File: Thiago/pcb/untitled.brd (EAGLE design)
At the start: 87.1 x 59.9 mm, 22 parts, among them IC1 LM358N, J3 -, J5 -

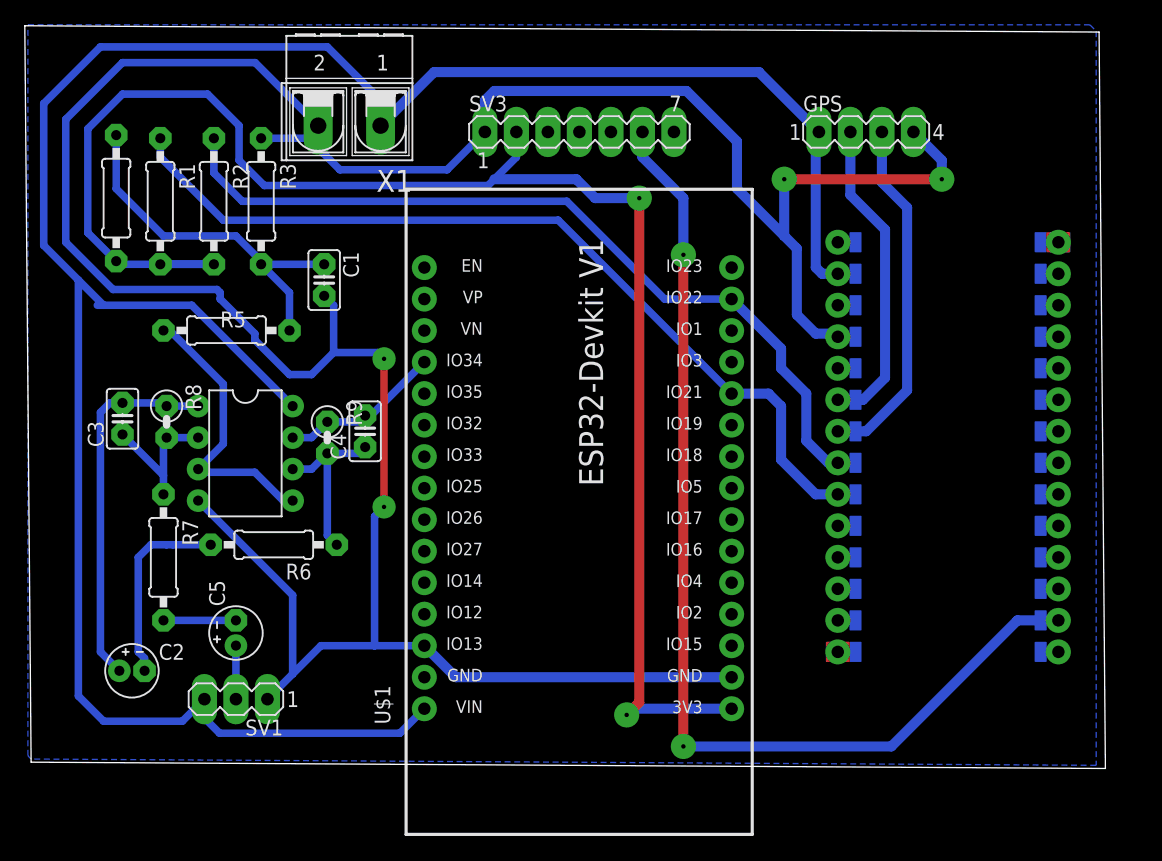
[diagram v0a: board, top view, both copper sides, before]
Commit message: Corrigi espaçãmento pcb
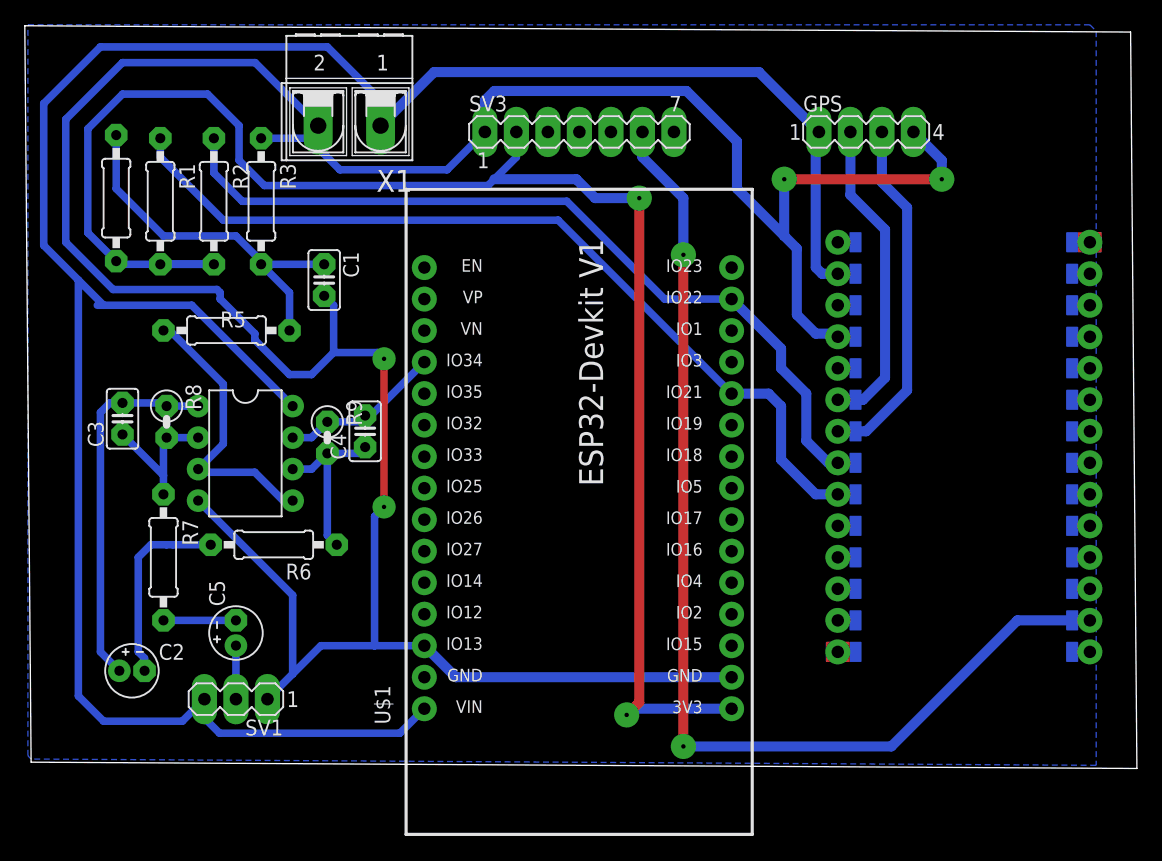
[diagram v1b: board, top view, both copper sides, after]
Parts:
- moved J3 2.54 mm to (100.3, 83.8)
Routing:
- net PWM_OUT: track 85.3 -> 87.9 mm
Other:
- board size 87.1 x 59.9 mm -> 89.6 x 59.9 mm
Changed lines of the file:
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@@
 <setting verticaltext="up"/>
 </settings>
-<grid distance="10" unitdist="mil" unit="mil" style="lines" multiple="1" display="no" altdistance="5" altunitdist="mil" altunit="mil"/>
+<grid distance="0.1" unitdist="mm" unit="mm" style="lines" multiple="1" display="no" altdistance="5" altunitdist="mil" altunit="mil"/>
 <layers>
-<layer number="1" name="Top" color="4" fill="1" visible="yes" active="yes"/>
+<layer number="1" name="Top" color="4" fill="1" visible="no" active="yes"/>
 <layer number="2" name="Route2" color="16" fill="1" visible="no" active="no"/>
 <layer number="3" name="Route3" color="17" fill="1" visible="no" active="no"/>
@@
 <layer number="17" name="Pads" color="2" fill="1" visible="yes" active="yes"/>
 <layer number="18" name="Vias" color="2" fill="1" visible="yes" active="yes"/>
-<layer number="19" name="Unrouted" color="6" fill="1" visible="yes" active="yes"/>
-<layer number="20" name="Dimension" color="24" fill="1" visible="yes" active="yes"/>
-<layer number="21" name="tPlace" color="7" fill="1" visible="yes" active="yes"/>
+<layer number="19" name="Unrouted" color="6" fill="1" visible="no" active="yes"/>
+<layer number="20" name="Dimension" color="24" fill="1" visible="no" active="yes"/>
+<layer number="21" name="tPlace" color="7" fill="1" visible="no" active="yes"/>
 <layer number="22" name="bPlace" color="7" fill="1" visible="no" active="yes"/>
 <layer number="23" name="tOrigins" color="15" fill="1" visible="no" active="yes"/>
@@
 <board>
 <plain>
-<wire x1="14.986" y1="41.91" x2="101.58" y2="41.402" width="0" layer="20"/>
-<wire x1="101.58" y1="41.402" x2="101.072" y2="100.762" width="0" layer="20"/>
-<wire x1="101.072" y1="100.762" x2="14.478" y2="101.27" width="0" layer="20"/>
+<wire x1="14.986" y1="41.91" x2="104.12" y2="41.402" width="0" layer="20"/>
+<wire x1="104.12" y1="41.402" x2="103.612" y2="100.762" width="0" layer="20"/>
+<wire x1="103.612" y1="100.762" x2="14.478" y2="101.27" width="0" layer="20"/>
 <wire x1="14.478" y1="101.27" x2="14.986" y2="41.91" width="0" layer="20"/>
+<dimension x1="101.58" y1="41.402" x2="101.072" y2="100.762" x3="104.357475" y3="71.107940625" textsize="1.778" layer="1"/>
 </plain>
 <attributes>
@@
 </autorouter>
 <elements>
-<element name="J3" library="Arduino-connectors" package="1X14_SMD_TH" value="-" x="97.79" y="83.82" smashed="yes" rot="R270">
-<attribute name="DATASHEET" value="-" x="60.96" y="26.67" size="1.778" layer="27" rot="R270" display="off"/>
-<attribute name="DISTRIBUTOR-LINK" value="-" x="60.96" y="26.67" size="1.778" layer="27" rot="R270" display="off"/>
-<attribute name="DISTRIBUTOR-PN" value="-" x="60.96" y="26.67" size="1.778" layer="27" rot="R270" display="off"/>
-<attribute name="MANUFACTURER" value="ELDECO" x="60.96" y="26.67" size="1.778" layer="27" rot="R270" display="off"/>
-<attribute name="MANUFACTURER-PN" value="FH254114DF08500T" x="60.96" y="26.67" size="1.778" layer="27" rot="R270" display="off"/>
-<attribute name="NAME" x="100.33" y="85.09" size="1.2" layer="25" font="vector" ratio="10" rot="R270"/>
-<attribute name="NAME" x="99.06" y="82.55" size="0.92" layer="51" font="vector" ratio="10" rot="R270"/>
-<attribute name="VALUE" x="97.79" y="82.55" size="1.2" layer="27" font="vector" ratio="10" rot="R270"/>
+<element name="J3" library="Arduino-connectors" package="1X14_SMD_TH" value="-" x="100.33" y="83.82" smashed="yes" rot="R270">
+<attribute name="DATASHEET" value="-" x="63.5" y="26.67" size="1.778" layer="27" rot="R270" display="off"/>
+<attribute name="DISTRIBUTOR-LINK" value="-" x="63.5" y="26.67" size="1.778" layer="27" rot="R270" display="off"/>
+<attribute name="DISTRIBUTOR-PN" value="-" x="63.5" y="26.67" size="1.778" layer="27" rot="R270" display="off"/>
+<attribute name="MANUFACTURER" value="ELDECO" x="63.5" y="26.67" size="1.778" layer="27" rot="R270" display="off"/>
+<attribute name="MANUFACTURER-PN" value="FH254114DF08500T" x="63.5" y="26.67" size="1.778" layer="27" rot="R270" display="off"/>
+<attribute name="NAME" x="102.87" y="85.09" size="1.2" layer="25" font="vector" ratio="10" rot="R270"/>
+<attribute name="NAME" x="101.6" y="82.55" size="0.92" layer="51" font="vector" ratio="10" rot="R270"/>
+<attribute name="VALUE" x="100.33" y="82.55" size="1.2" layer="27" font="vector" ratio="10" rot="R270"/>
 </element>
 <element name="J5" library="Arduino-connectors" package="1X14_SMD_TH" value="-" x="80.01" y="50.8" smashed="yes" rot="R90">
@@
 <via x="67.564" y="43.18" extent="1-16" drill="0.35" diameter="2.032"/>
 <wire x1="67.564" y1="43.18" x2="84.328" y2="43.18" width="0.8128" layer="16"/>
-<wire x1="94.488" y1="53.34" x2="97.79" y2="53.34" width="0.8128" layer="16"/>
+<wire x1="94.488" y1="53.34" x2="100.33" y2="53.34" width="0.8128" layer="16"/>
 <wire x1="84.328" y1="43.18" x2="94.488" y2="53.34" width="0.8128" layer="16"/>
 </signal>
